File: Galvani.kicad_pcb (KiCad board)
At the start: 4 copper layers, 127 x 38.1 mm, 123 parts, among them J1 USB-C Receptacle, J2 U.FL Connector, J3 JST-PH-1x3, J4 JST-PH-1x3, J5 JST PH2.0-1x2, J6 JST PH2.0-1x2, J8 Micro SD Card, P1 Cap 2.4pF 0201, P2 L 2.7nH 0201, P3 Cap 3.9pF 0201, P7 L 2.7nH 0201, SW1 Pushbutton 4.2x3.2mm 250gf, SW2 Pushbutton 4.2x3.2mm 250gf, U1 LMR14030SDDAR, U10 MEMS Microphone, U2 ESP32-S3, U3 W25Q128JVS, U4 SN74LVC1T45DBVR, U5 TPS560430, U6 SN74LVC1T45DBVR, U7 ES7149, U8 NS4150, U9 NS4150, Y1 Crystal 40MHz 2016

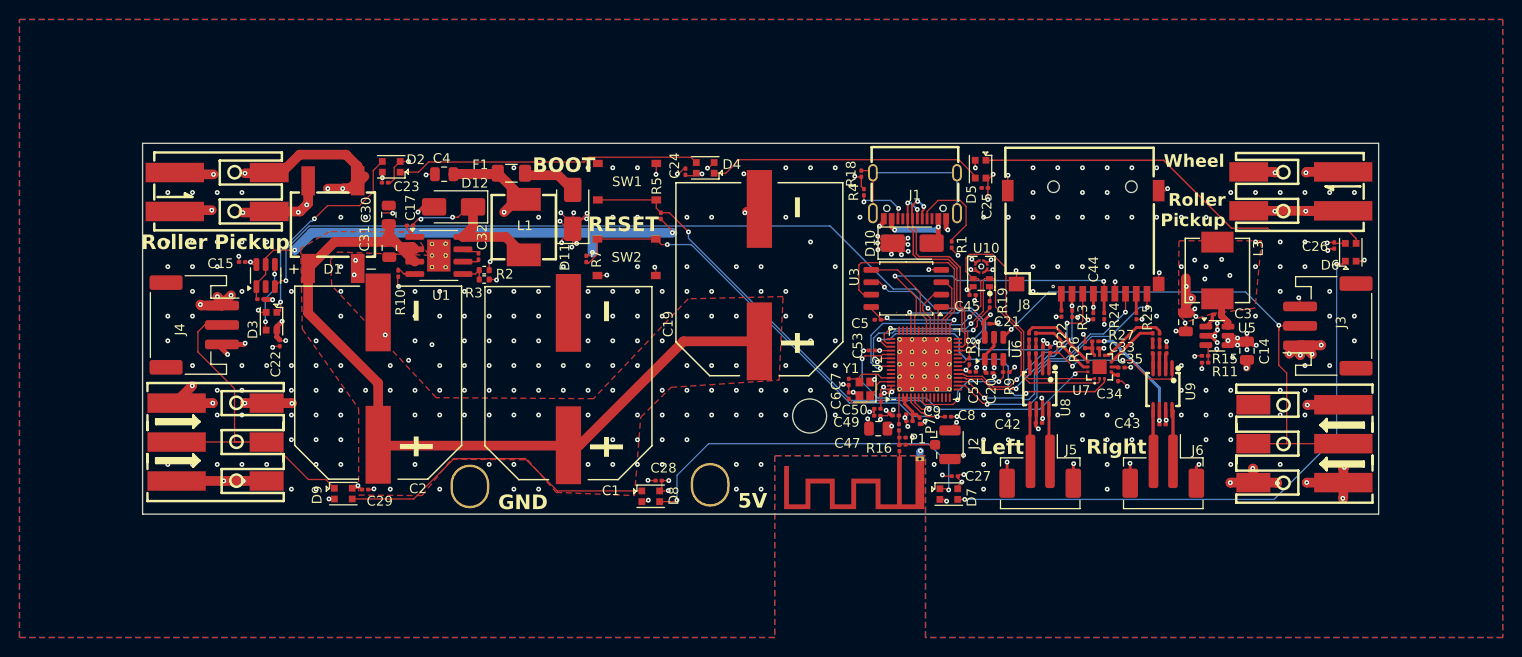
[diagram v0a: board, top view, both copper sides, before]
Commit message: release evt2
Signed-off-by: Sean Cross <sean@xobs.io>
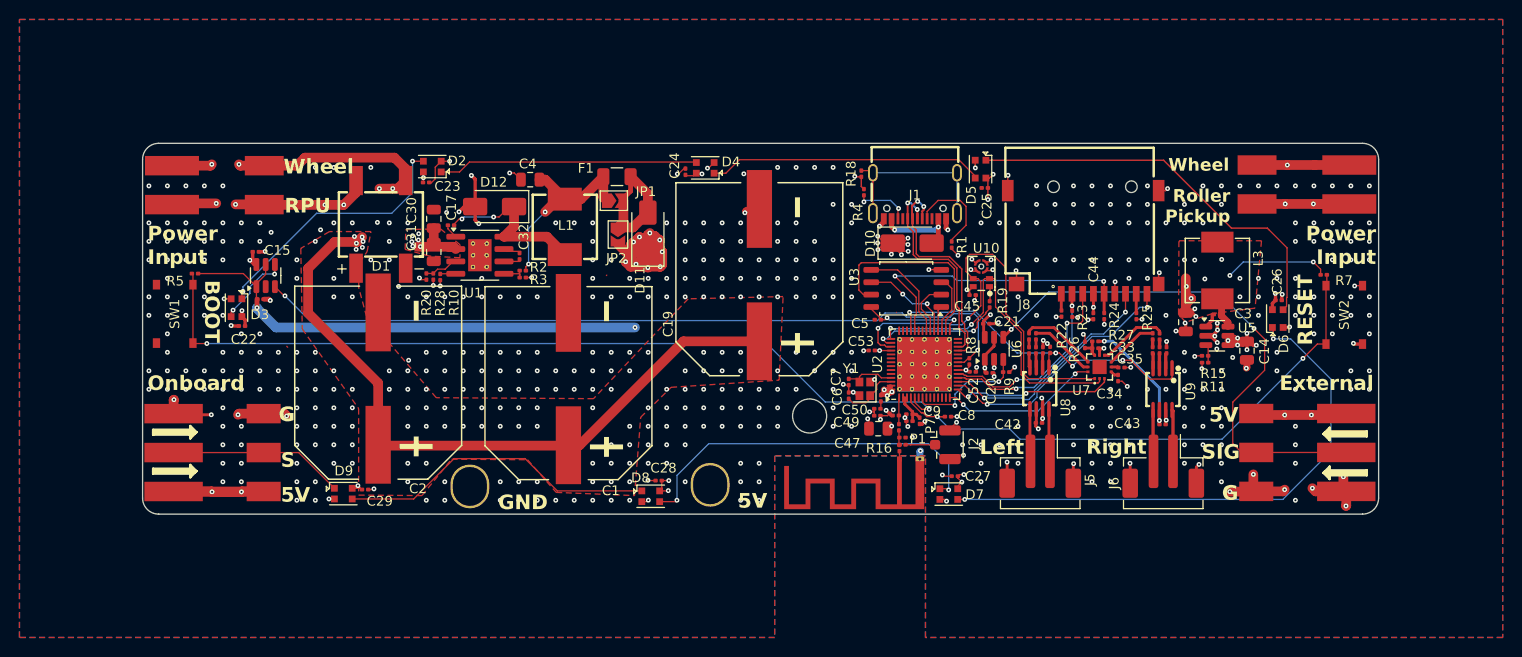
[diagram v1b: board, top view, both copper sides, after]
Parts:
- removed J3, J4: JST-PH-1x3, Connector_JST:JST_PH_S3B-PH-SM4-TB_1x03-1MP_P2.00mm_Horizontal
- removed kibuzzard-66F0D9BF: G***, kibuzzard-66F0D9BF
- added JP1: Fuse Bypass, Jumper:SolderJumper-2_P1.3mm_Open_TrianglePad1.0x1.5mm, F.Cu at (128.7, 89.1)
- added JP2: Fuse Bypass, Jumper:SolderJumper-2_P1.3mm_Open_TrianglePad1.0x1.5mm, F.Cu at (129.1, 92.6)
- added R20: R 140k 0201, Galvani:R_0201_0603Metric, F.Cu at (109.4, 96.9)
- added R28: R 34k 0201, Galvani:R_0201_0603Metric, F.Cu at (110.1, 96.9)
- added kibuzzard-67065BC0: G***, kibuzzard-67065BC0, B.Cu at (141.9, 96.5)
- D2, D3, D4, D5, D6, D7, D8, D9: value WS2812C-2020 -> WS2812B-2020
- R10, R12, R13, R14, R21, R22, R23, R24, R25, R5, R6, R7, R8, R9: value R 20k 0201 -> R 22.1k 0201
- R2: value R 68k 0402 -> R 68k 0201; footprint Resistor_SMD:R_0402_1005Metric -> Galvani:R_0201_0603Metric
- R3: value R 12k 0402 -> R 12k 0201; footprint Resistor_SMD:R_0402_1005Metric -> Galvani:R_0201_0603Metric
- moved R7 75.8 mm to (201.6, 96.7), turned to 0 degrees
- moved SW2 74.0 mm to (203.7, 100.8), turned to -90 degrees
- moved SW1 48.4 mm to (83.6, 100.7), turned to 90 degrees
- moved R5 48.2 mm to (85.6, 96.6), turned to 180 degrees
- moved F1 10.9 mm to (129.0, 86.6)
- moved D6 10.1 mm to (196.9, 101.2)
- moved C4 8.86 mm to (120.1, 86.9)
- moved D11 8.07 mm to (132.2, 92.3)
- moved C26 8.01 mm to (197.0, 99.3), turned to 0 degrees
- moved D1 4.93 mm to (104.7, 91.5)
- moved C30 4.64 mm to (110.2, 90.9)
- moved C31 4.59 mm to (110.2, 94.4)
- moved R10 4.33 mm to (110.8, 96.9)
- moved C22 4.27 mm to (90.5, 102.0), turned to 180 degrees
- moved C17 4.22 mm to (112.0, 91.6)
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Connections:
- CONN1 pad 1: V5V -> GND
- CONN1 pad 3: GND -> V5V
- CONN2 pad 1: V5V -> GND
- CONN2 pad 3: GND -> V5V
- TP1 pad 1: V5V -> GND
- TP2 pad 1: GND -> V5V
- U1 pad 3: /Heirarchy/Power/VAC_RECTIFIED -> Net-(U1-EN)
- U2 pad 14: unconnected-(U2-GPIO9/ADC1_CH8-Pad14) -> /Heirarchy/Audio/I2S_OUT
- U2 pad 15: unconnected-(U2-GPIO10/ADC1_CH9-Pad15) -> /Heirarchy/Audio/I2S_MCLK
- U2 pad 43: unconnected-(U2-GPIO38-Pad43) -> /Heirarchy/Audio/I2S_LRCK
- U2 pad 44: /Heirarchy/Audio/I2S_LRCK -> /Heirarchy/Audio/I2S_IN
- U2 pad 45: /Heirarchy/Audio/I2S_MCLK -> /Heirarchy/Audio/I2S_BCLK
- U2 pad 47: /Heirarchy/Audio/I2S_OUT -> unconnected-(U2-MTDI/JTAG/GPIO41-Pad47)
- U2 pad 48: /Heirarchy/Audio/I2S_IN -> unconnected-(U2-MTMS/JTAG/GPIO42-Pad48)
- U2 pad 50: /Heirarchy/Audio/I2S_BCLK -> unconnected-(U2-U0RXD/PROG/GPIO44-Pad50)
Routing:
- net /Heirarchy/CPU/BOOT_MODE: track 46.1 -> 87.7 mm
- net /Heirarchy/Audio/I2S_OUT: track 31.5 -> 16.4 mm
- net Net-(D9-DOUT): track 34.1 -> 19.3 mm
- net /Heirarchy/Audio/I2S_MCLK: track 30.7 -> 16.5 mm
- net VWIFI: track 113.4 -> 126.6 mm
- net GND: track 100.1 -> 111.5 mm, vias 356 -> 566
- net Earth: track 141.3 -> 150.1 mm
- net Net-(D11-A): track 5.61 -> 14.0 mm
- net /Heirarchy/CPU/LED_INTERNAL: track 87.2 -> 80.3 mm
- net /Heirarchy/CPU/RESET: track 51.0 -> 57.3 mm
- net Net-(D2-DIN): track 21.7 -> 27.0 mm
- net Net-(D2-DOUT): track 31.3 -> 26.6 mm
- net V5V: track 111.4 -> 107.1 mm, vias 56 -> 43
- net /Heirarchy/Audio/I2S_IN: track 17.7 -> 13.6 mm
- net /Heirarchy/Audio/AUDIO_EN: track 39.5 -> 35.5 mm
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- added copper zone on In2.Cu, net /Heirarchy/Power/VAC_RECTIFIED
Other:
- outline, holes or cut-outs redrawn
- board text added: "Power Input"
- board text added: "RPU"
- board text added: "S"
